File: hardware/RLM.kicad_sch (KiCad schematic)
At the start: 12 parts, among them U6 AP1117-33

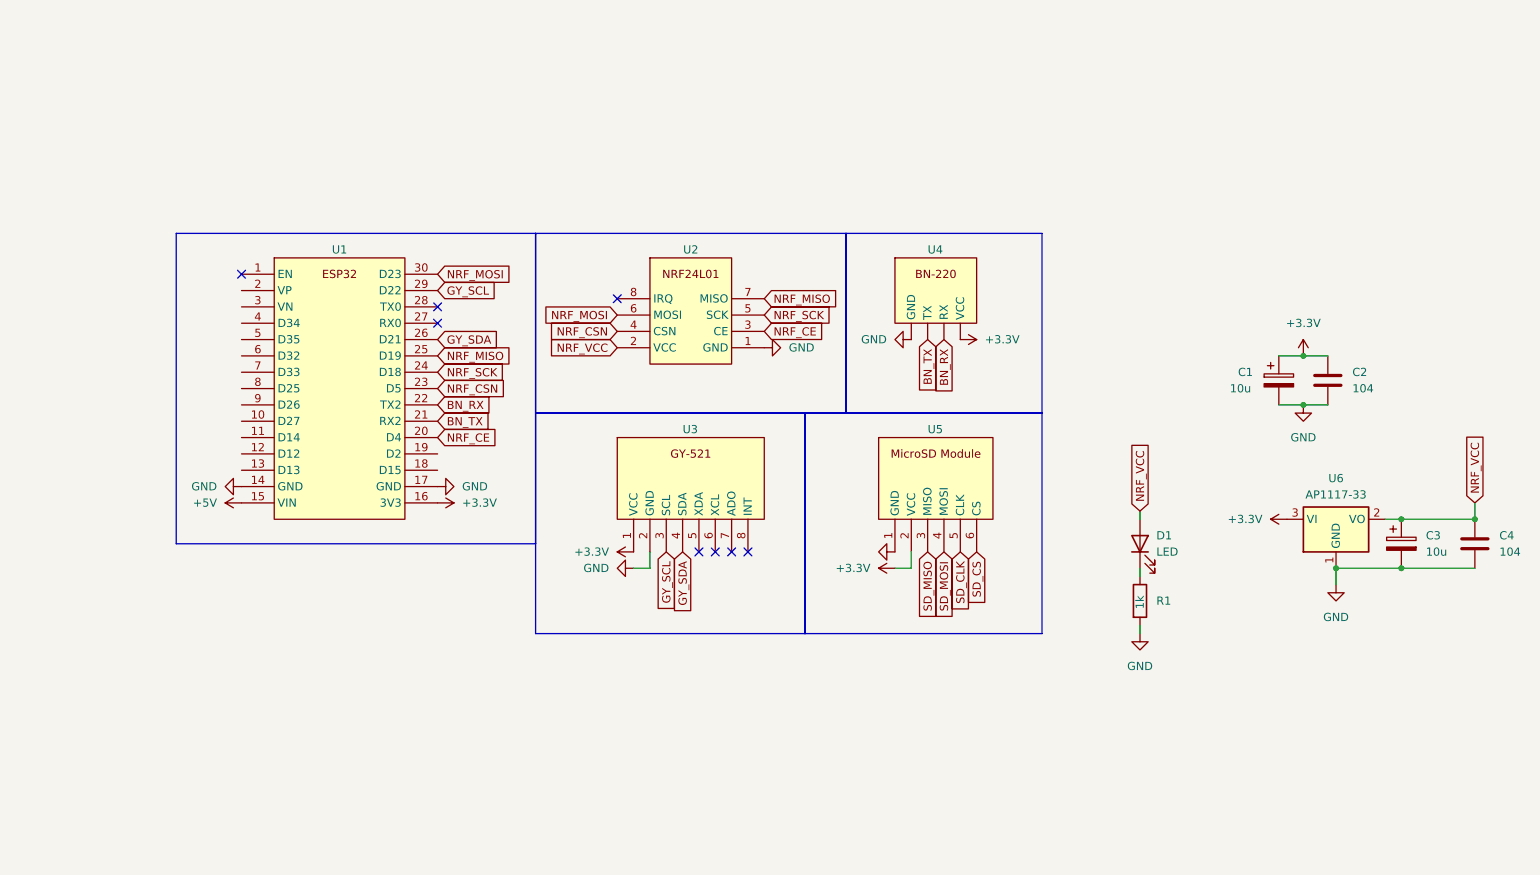
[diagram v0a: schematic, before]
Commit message: chore: reorganize schematic
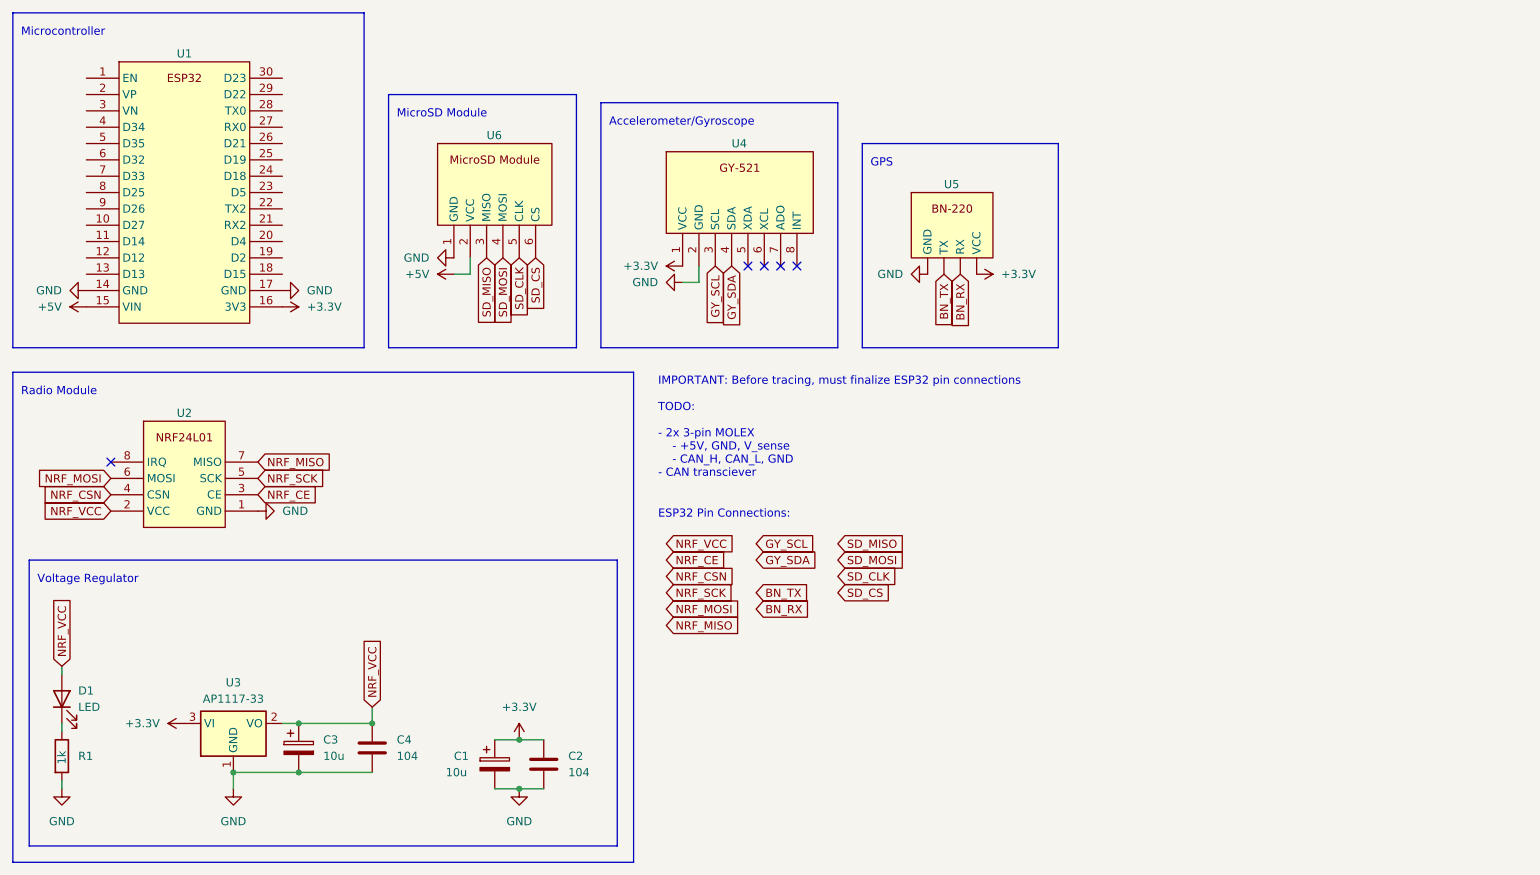
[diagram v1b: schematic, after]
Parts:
- renumbered U6 to U3, U3 to U4, U4 to U5, U5 to U6
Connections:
- net +3.3V: no longer U6.2 (VCC)
- net +5V: now also U6.2 (VCC)
- net BN_RX: no longer U1.22 (TX2)
- net BN_TX: no longer U1.21 (RX2)
- net GY_SCL: no longer U1.29 (D22)
- net GY_SDA: no longer U1.26 (D21)
- net NRF_CE: no longer U1.20 (D4)
- net NRF_CSN: no longer U1.23 (D5)
- net NRF_MISO: no longer U1.25 (D19)
- net NRF_MOSI: no longer U1.30 (D23)
- net NRF_SCK: no longer U1.24 (D18)
- no-connect marks 8 -> 5
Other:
- note added: "Accelerometer/Gyroscope"
- note added: "ESP32 Pin Connections:"
- note added: "GPS"
- note added: "IMPORTANT: Before tracing, must finalize ESP32 pin connections TODO: - 2x 3-pin MOLEX - +5V, GND, V_sense - CAN_H, CAN_L, GND - CAN transciever"
- note added: "MicroSD Module"
- note added: "Microcontroller"
- note added: "Radio Module"
- note added: "Voltage Regulator"
- title: (none) -> Remote Logging Module
- moved on the sheet: C1, C2, C3, C4, D1, R1, U1, U2, U3, U4, U5, U6
